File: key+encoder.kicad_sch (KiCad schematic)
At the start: 2 parts, among them SW10 SW_Push

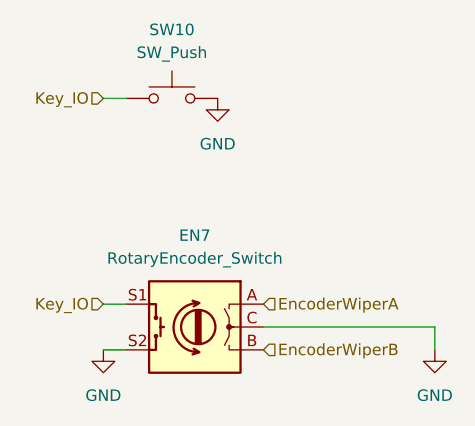
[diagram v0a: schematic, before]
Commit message: updated libs, positioned jumpers
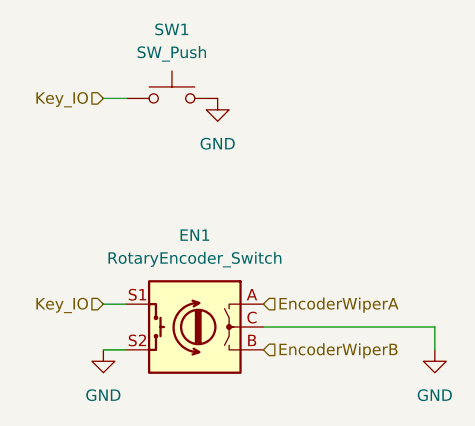
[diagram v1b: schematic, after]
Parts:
- renumbered EN7 to EN1, SW10 to SW1
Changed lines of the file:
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@@
   (symbol (lib_id "power:GND") (at 146.05 96.52 0)
     (in_bom yes) (on_board yes) (fields_autoplaced)
-    (property "Reference" "#PWR020" (id 0) (at 146.05 102.87 0)
+    (property "Reference" "#PWR02" (id 0) (at 146.05 102.87 0)
       (effects (font (size 1.27 1.27)) hide)
     )
@@
   (symbol (lib_id "power:GND") (at 170.18 124.46 0)
     (in_bom yes) (on_board yes) (fields_autoplaced)
-    (property "Reference" "#PWR021" (id 0) (at 170.18 130.81 0)
+    (property "Reference" "#PWR03" (id 0) (at 170.18 130.81 0)
       (effects (font (size 1.27 1.27)) hide)
     )
@@
   (symbol (lib_id "Device:RotaryEncoder_Switch") (at 143.51 121.92 0) (mirror y)
     (in_bom yes) (on_board yes) (fields_autoplaced)
-    (property "Reference" "EN7" (id 0) (at 143.51 111.76 0))
+    (property "Reference" "EN1" (id 0) (at 143.51 111.76 0))
     (property "Value" "RotaryEncoder_Switch" (id 1) (at 143.51 114.3 0))
     (property "Footprint" "Keeby-Cat Footprints:RotaryEncoder_Alps_EC11E-Switch_Vertical_H20mm_nomount_alt" (id 2) (at 147.32 117.856 0)
@@
   (symbol (lib_id "power:GND") (at 133.35 124.46 0)
     (in_bom yes) (on_board yes) (fields_autoplaced)
-    (property "Reference" "#PWR019" (id 0) (at 133.35 130.81 0)
+    (property "Reference" "#PWR01" (id 0) (at 133.35 130.81 0)
       (effects (font (size 1.27 1.27)) hide)
     )
@@
   (symbol (lib_id "Switch:SW_Push") (at 140.97 96.52 0)
     (in_bom yes) (on_board yes) (fields_autoplaced)
-    (property "Reference" "SW10" (id 0) (at 140.97 88.9 0))
+    (property "Reference" "SW1" (id 0) (at 140.97 88.9 0))
     (property "Value" "SW_Push" (id 1) (at 140.97 91.44 0))
     (property "Footprint" "kbd-footprints:CherryMX_1u_north" (id 2) (at 140.97 91.44 0)

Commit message: initial board routing
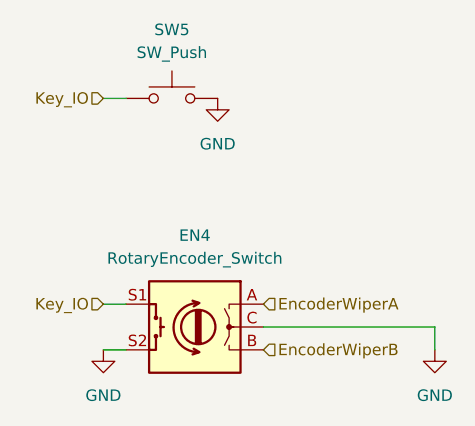
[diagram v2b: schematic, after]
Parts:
- renumbered EN1 to EN4, SW1 to SW5
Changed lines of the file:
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@@
   (symbol (lib_id "power:GND") (at 146.05 96.52 0)
     (in_bom yes) (on_board yes) (fields_autoplaced)
-    (property "Reference" "#PWR02" (id 0) (at 146.05 102.87 0)
+    (property "Reference" "#PWR011" (id 0) (at 146.05 102.87 0)
       (effects (font (size 1.27 1.27)) hide)
     )
@@
   (symbol (lib_id "power:GND") (at 170.18 124.46 0)
     (in_bom yes) (on_board yes) (fields_autoplaced)
-    (property "Reference" "#PWR03" (id 0) (at 170.18 130.81 0)
+    (property "Reference" "#PWR012" (id 0) (at 170.18 130.81 0)
       (effects (font (size 1.27 1.27)) hide)
     )
@@
   (symbol (lib_id "Device:RotaryEncoder_Switch") (at 143.51 121.92 0) (mirror y)
     (in_bom yes) (on_board yes) (fields_autoplaced)
-    (property "Reference" "EN1" (id 0) (at 143.51 111.76 0))
+    (property "Reference" "EN4" (id 0) (at 143.51 111.76 0))
     (property "Value" "RotaryEncoder_Switch" (id 1) (at 143.51 114.3 0))
     (property "Footprint" "Keeby-Cat Footprints:RotaryEncoder_Alps_EC11E-Switch_Vertical_H20mm_nomount_alt" (id 2) (at 147.32 117.856 0)
@@
   (symbol (lib_id "power:GND") (at 133.35 124.46 0)
     (in_bom yes) (on_board yes) (fields_autoplaced)
-    (property "Reference" "#PWR01" (id 0) (at 133.35 130.81 0)
+    (property "Reference" "#PWR010" (id 0) (at 133.35 130.81 0)
       (effects (font (size 1.27 1.27)) hide)
     )
@@
   (symbol (lib_id "Switch:SW_Push") (at 140.97 96.52 0)
     (in_bom yes) (on_board yes) (fields_autoplaced)
-    (property "Reference" "SW1" (id 0) (at 140.97 88.9 0))
+    (property "Reference" "SW5" (id 0) (at 140.97 88.9 0))
     (property "Value" "SW_Push" (id 1) (at 140.97 91.44 0))
     (property "Footprint" "kbd-footprints:CherryMX_1u_north" (id 2) (at 140.97 91.44 0)

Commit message: shrank board outline to 100mm max
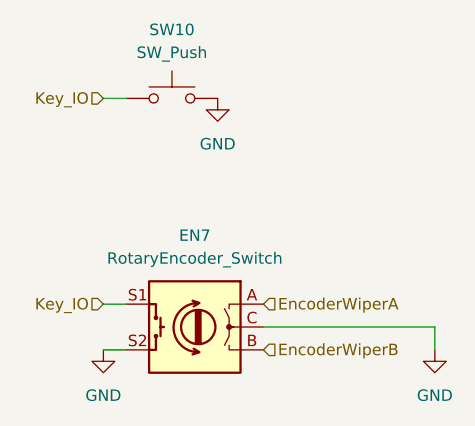
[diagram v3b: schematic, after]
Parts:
- renumbered EN4 to EN7, SW5 to SW10
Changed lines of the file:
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@@
   (symbol (lib_id "power:GND") (at 146.05 96.52 0)
     (in_bom yes) (on_board yes) (fields_autoplaced)
-    (property "Reference" "#PWR011" (id 0) (at 146.05 102.87 0)
+    (property "Reference" "#PWR020" (id 0) (at 146.05 102.87 0)
       (effects (font (size 1.27 1.27)) hide)
     )
@@
   (symbol (lib_id "power:GND") (at 170.18 124.46 0)
     (in_bom yes) (on_board yes) (fields_autoplaced)
-    (property "Reference" "#PWR012" (id 0) (at 170.18 130.81 0)
+    (property "Reference" "#PWR021" (id 0) (at 170.18 130.81 0)
       (effects (font (size 1.27 1.27)) hide)
     )
@@
   (symbol (lib_id "Device:RotaryEncoder_Switch") (at 143.51 121.92 0) (mirror y)
     (in_bom yes) (on_board yes) (fields_autoplaced)
-    (property "Reference" "EN4" (id 0) (at 143.51 111.76 0))
+    (property "Reference" "EN7" (id 0) (at 143.51 111.76 0))
     (property "Value" "RotaryEncoder_Switch" (id 1) (at 143.51 114.3 0))
     (property "Footprint" "Keeby-Cat Footprints:RotaryEncoder_Alps_EC11E-Switch_Vertical_H20mm_nomount_alt" (id 2) (at 147.32 117.856 0)
@@
   (symbol (lib_id "power:GND") (at 133.35 124.46 0)
     (in_bom yes) (on_board yes) (fields_autoplaced)
-    (property "Reference" "#PWR010" (id 0) (at 133.35 130.81 0)
+    (property "Reference" "#PWR019" (id 0) (at 133.35 130.81 0)
       (effects (font (size 1.27 1.27)) hide)
     )
@@
   (symbol (lib_id "Switch:SW_Push") (at 140.97 96.52 0)
     (in_bom yes) (on_board yes) (fields_autoplaced)
-    (property "Reference" "SW5" (id 0) (at 140.97 88.9 0))
+    (property "Reference" "SW10" (id 0) (at 140.97 88.9 0))
     (property "Value" "SW_Push" (id 1) (at 140.97 91.44 0))
     (property "Footprint" "kbd-footprints:CherryMX_1u_north" (id 2) (at 140.97 91.44 0)
